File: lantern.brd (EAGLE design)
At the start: 50 x 40 mm, 39 parts, among them T1 2N2222B, T2 2N2222B, T3 2N2222B, T4_2SC2120Y 2N2222B, T5_2SA950 2N2907, U2 HT7733A

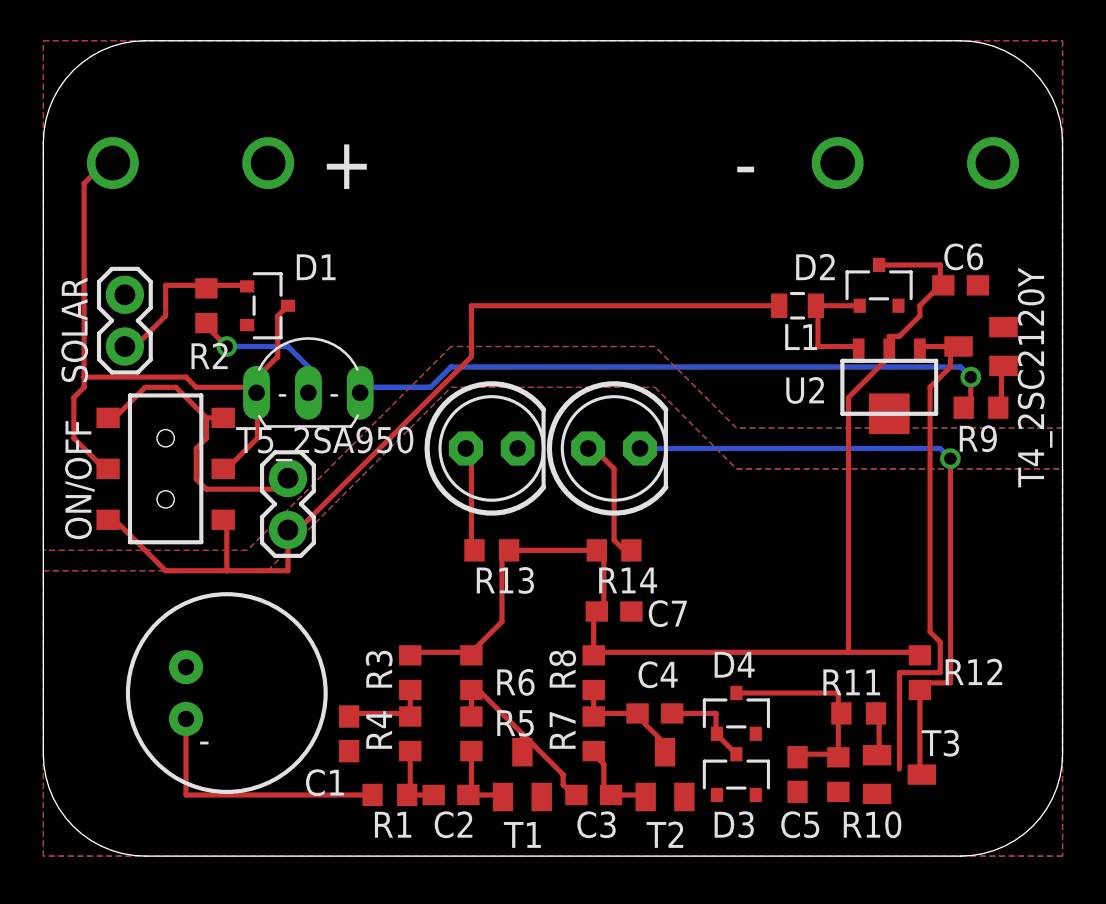
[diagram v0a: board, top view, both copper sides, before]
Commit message: RevA pcb finished, first case version
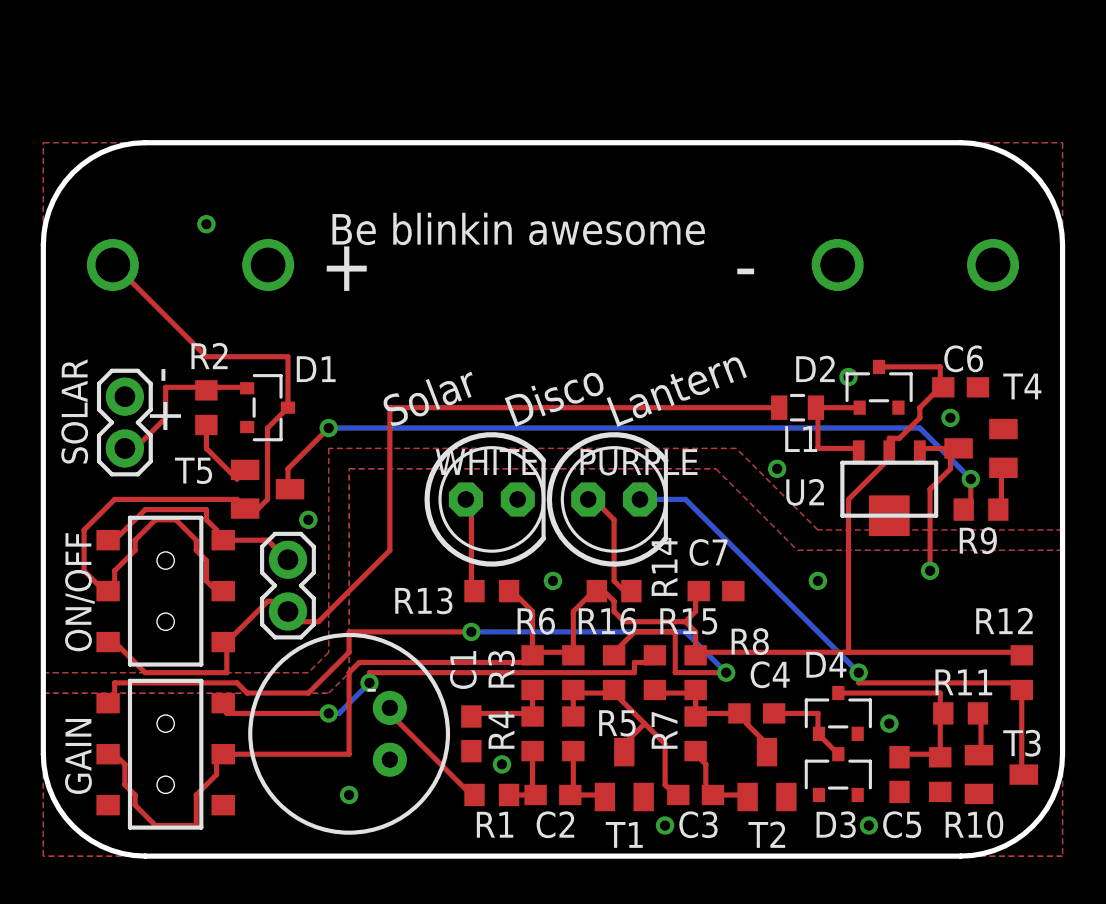
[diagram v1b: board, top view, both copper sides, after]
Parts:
- removed T4_2SC2120Y: 2N2222B, blinkinlabs:SOT23
- removed T5_2SA950: 2N2907, adafruit:TO92-EBC-OVAL
- added GAIN: AYZ0202, SparkFun-Electromechanical:AYZ0202
- added R15, R16: 15K, adafruit:R0603
- added T4: 2N2222B, blinkinlabs:SOT23
- added T5: 2N2907B, blinkinlabs:SOT23
- moved U$1 6.32 mm to (15.0, 6.00), turned to 180 degrees
- moved C1 6.00 mm to (21.0, 6.00)
- moved ON/OFF 6.00 mm to (6.00, 13.0)
- moved R3 6.00 mm to (24.0, 9.00)
- moved R4 6.00 mm to (24.0, 6.00)
- moved C7 5.10 mm to (33.0, 13.0)
- moved BAT1 5.00 mm to (25.0, 29.0)
- moved C2 5.00 mm to (25.0, 3.00)
- moved C3 5.00 mm to (32.0, 3.00)
- moved C4 5.00 mm to (35.0, 7.00)
- moved C5 5.00 mm to (42.0, 4.00)
- moved C6 5.00 mm to (45.0, 23.0)
- moved D1 5.00 mm to (11.0, 22.0)
- moved D2 5.00 mm to (41.0, 23.0)
- moved D3 5.00 mm to (39.0, 4.00)
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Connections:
- new net N$22: GAIN.4, R16.2
- new net N$23: GAIN.1, R15.2
- net DGND: now also T4.2; no longer T4_2SC2120Y.2
- net GND: now also T4.3; no longer T4_2SC2120Y.3
- net N$13: now also T5.3; no longer T5_2SA950.C
- net N$14: now also T4.1; no longer T4_2SC2120Y.1
- net N$15: now also T5.2; no longer T5_2SA950.E
- net N$16: now also T5.1; no longer T5_2SA950.B
- net N$4: now also R16.1
- net N$5: now also R15.1
- net VCC: now also GAIN.2, GAIN.5
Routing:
- net N$22: track 0.00 -> 42.3 mm, vias 0 -> 2
- net VCC: track 60.0 -> 84.5 mm
- net N$23: track 0.00 -> 23.6 mm, vias 0 -> 2
- net GND: track 25.5 -> 8.51 mm, vias 0 -> 8
- net N$15: track 35.0 -> 41.8 mm
- net N$7: track 12.9 -> 6.08 mm
- net N$13: track 32.5 -> 38.3 mm, vias 1 -> 2
- net N$8: track 32.5 -> 27.4 mm
- net N$21: track 15.3 -> 11.1 mm
- net N$16: track 7.25 -> 3.87 mm, vias 1 -> 0
- net N$5: track 6.11 -> 8.26 mm
- net N$4: track 10.3 -> 11.7 mm
- net N$17: track 44.9 -> 45.5 mm
- net N$20: track 6.24 -> 5.74 mm
- net N$19: track 5.42 -> 4.92 mm
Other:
- board size 50 x 40 mm -> 50 x 35 mm
- board text added: "Be blinkin awesome"
- board text added: "Disco"
- board text added: "Honghong"
- board text added: "Lantern"
- board text added: "Matt"
- board text added: "Solar"
- board text added: "and"
- board text removed: "Honghong and Matt"
